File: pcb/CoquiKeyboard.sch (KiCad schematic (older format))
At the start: 116 parts, among them SW1 SW_Push, U1 ATmega32U4-MU, Y1 16MHz

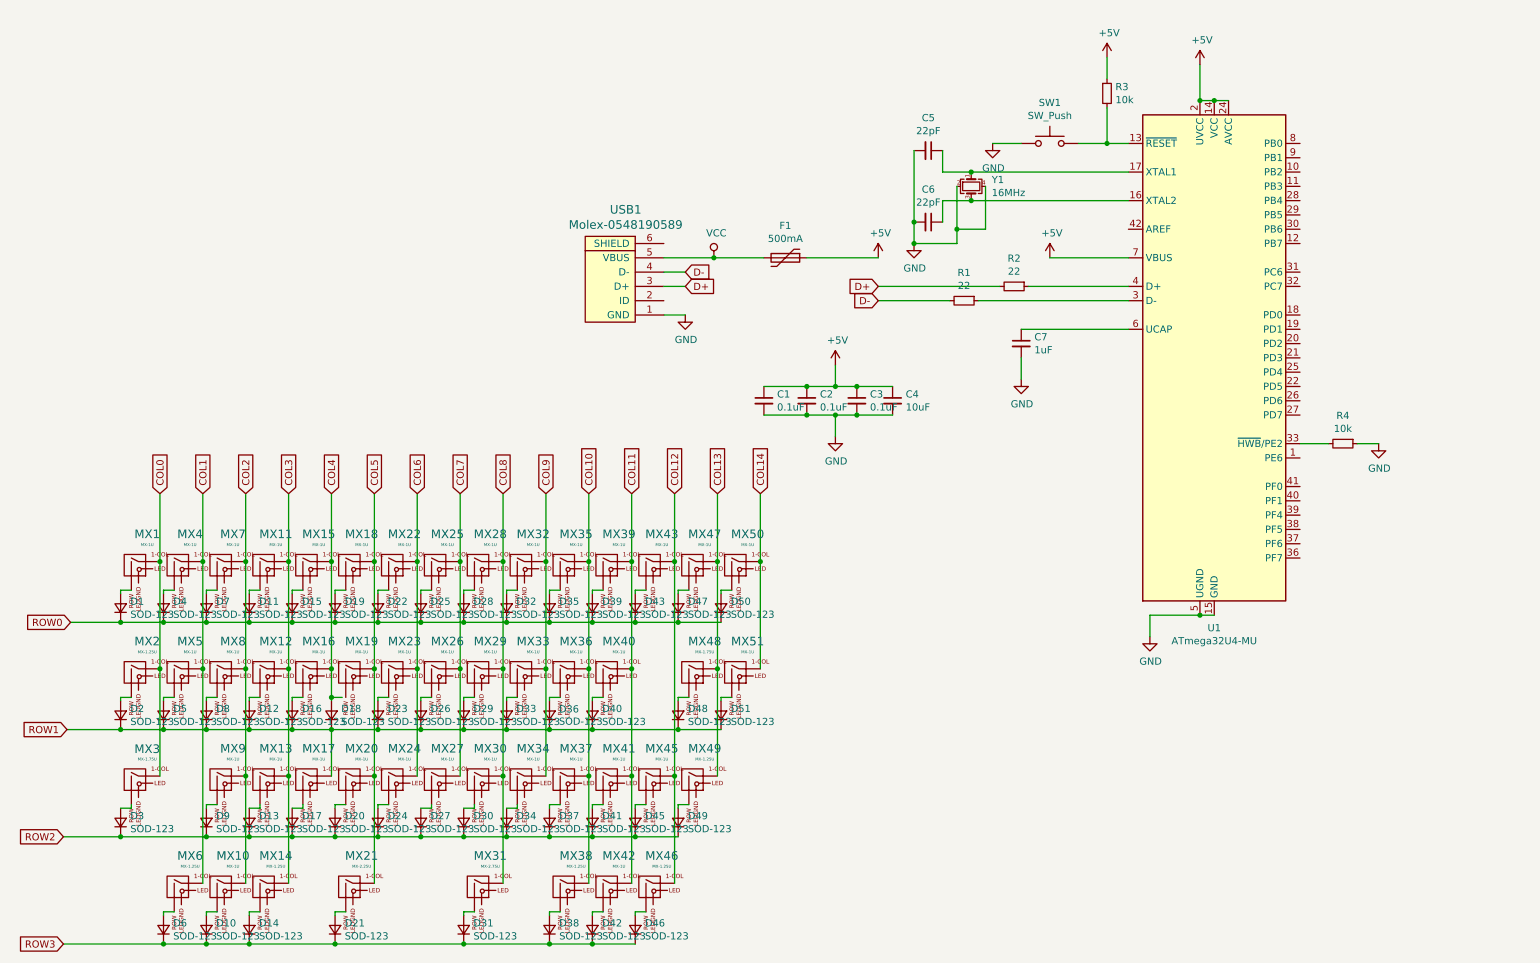
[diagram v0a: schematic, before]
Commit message: clean up ratsnet
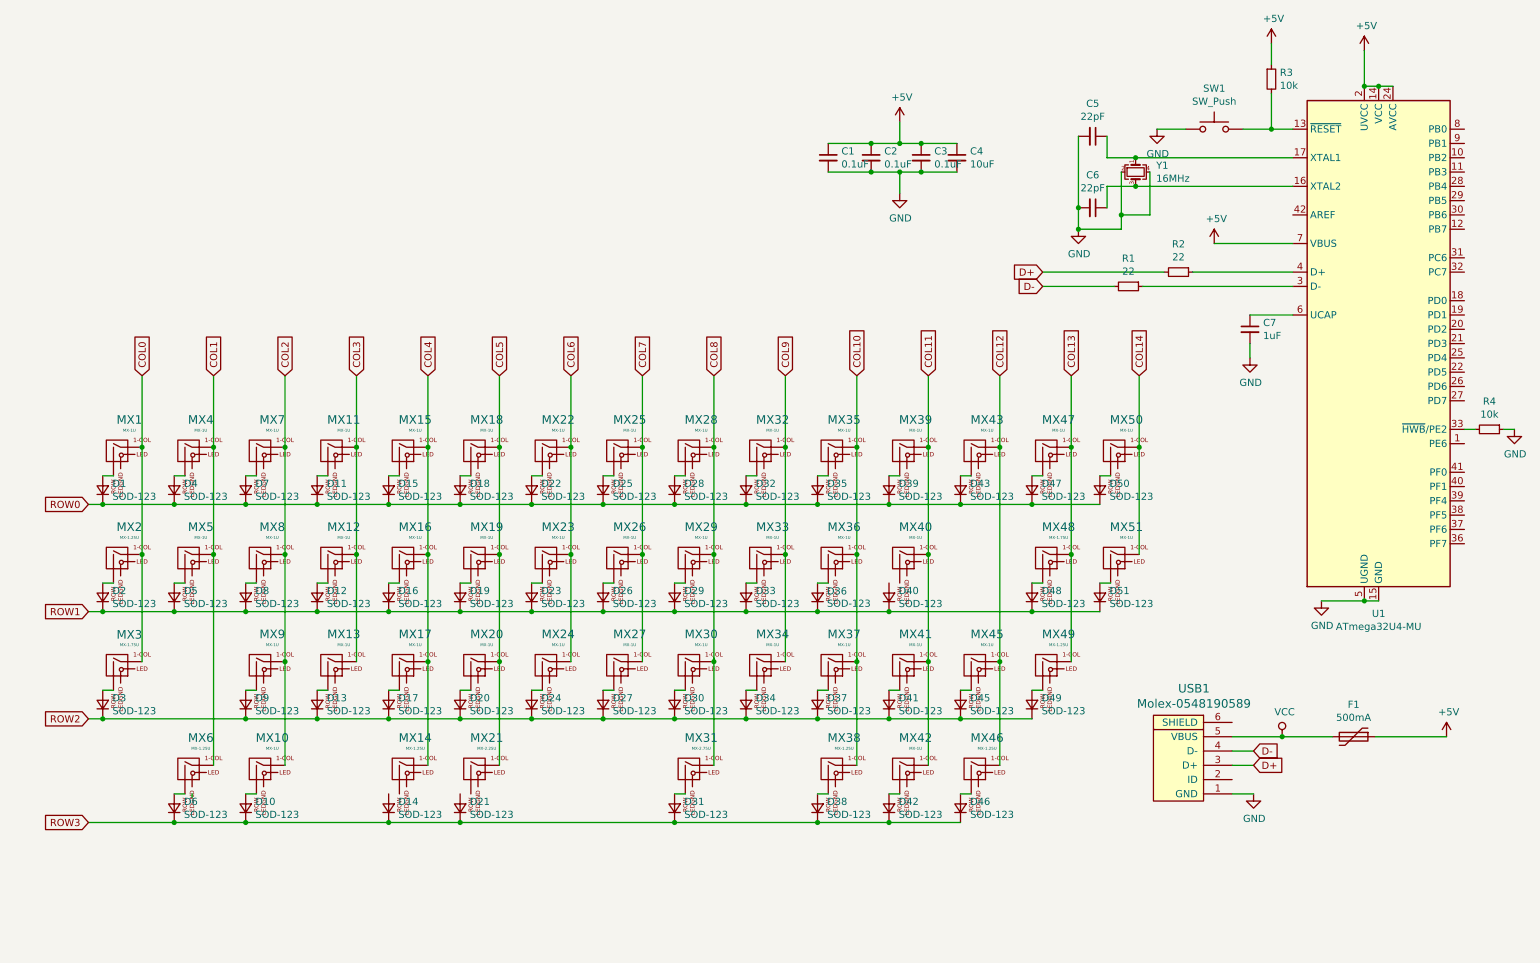
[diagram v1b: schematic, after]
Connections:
- net COL3: no longer MX14.1 (COL)
- net COL4: now also MX14.1 (COL), MX17.1 (COL); no longer D18.2 (A)
- net ROW0: now also D18.1 (K); no longer D19.1 (K)
- net ROW1: now also D19.1 (K); no longer D18.1 (K), MX17.1 (COL)
- net at MX18.2 (ROW): now also D18.2 (A); no longer D19.2 (A)
- net at MX19.2 (ROW): now also D19.2 (A)
- net at MX40.2 (ROW): no longer D40.2 (A)
- net at MX14.2 (ROW): no longer D14.2 (A)
- net at MX21.2 (ROW): no longer D21.2 (A)
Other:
- moved on the sheet: C1, C2, C3, C4, C5, C6, C7, D1, D10, D11, D12, D13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
